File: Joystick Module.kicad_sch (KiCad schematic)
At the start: 2 parts, among them J1 Conn_01x05_Pin

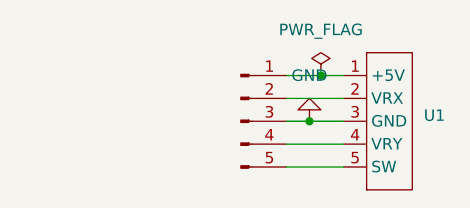
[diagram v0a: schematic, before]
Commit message: Add files via upload
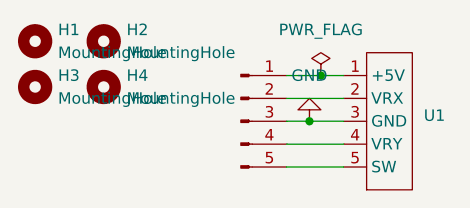
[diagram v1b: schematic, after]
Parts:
- added H1, H2, H3, H4: MountingHole, MountingHole:MountingHole_2.2mm_M2, symbol Mechanical:MountingHole
